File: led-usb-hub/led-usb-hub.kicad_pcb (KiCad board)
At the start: 4 copper layers, 58.4 x 38.7 mm, 126 parts, among them J1 USBC_USB2.0, J2 RGBUSB_54-00266, J3 RGBUSB_54-00266, J4 RGBUSB_54-00266, J5 SWD, SW1 RESET, SW2 BOOT, SW3 LED EN, U1 STM32L552CETx, U12 MAX809, U2 TUSB2046IBVF, U3 TLV62569PDDCR, U4 TLV62569PDDCR, U5 TPS2042D, U6 TPS2042D, Y1 KC2520Z8.00000C1KX00, Y2 KC2520Z6.00000C1GX00

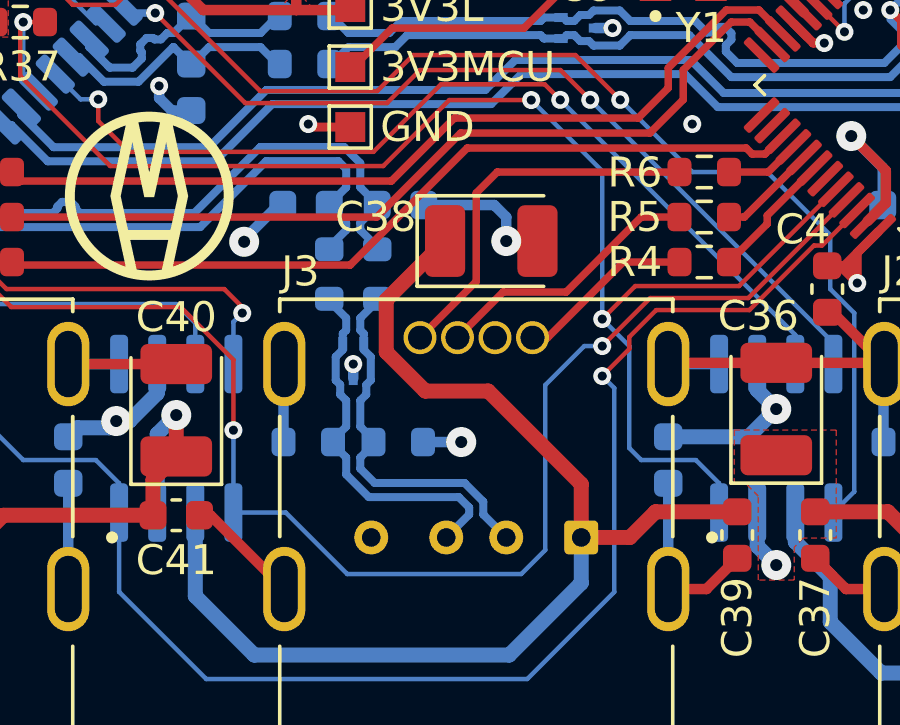
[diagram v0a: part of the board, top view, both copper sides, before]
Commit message: [HW] More Space
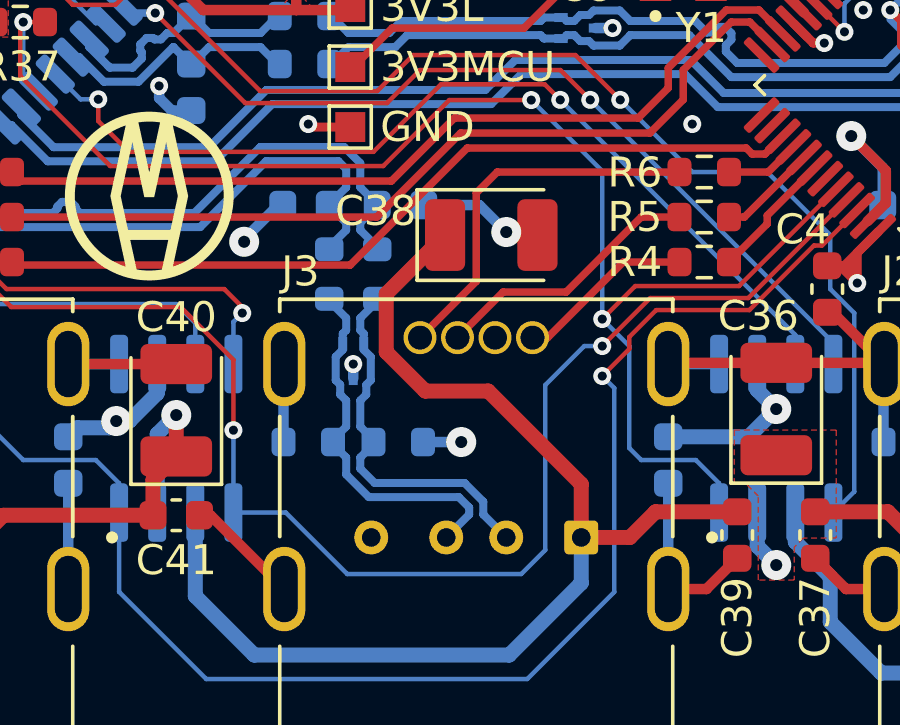
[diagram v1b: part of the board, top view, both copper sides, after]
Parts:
- moved C38 0.20 mm to (88.4, 93.1)
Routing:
- net Earth: track 193.8 -> 193.3 mm
